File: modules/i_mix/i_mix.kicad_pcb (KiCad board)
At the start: 2 copper layers, 30.5 x 68.6 mm, 4 parts

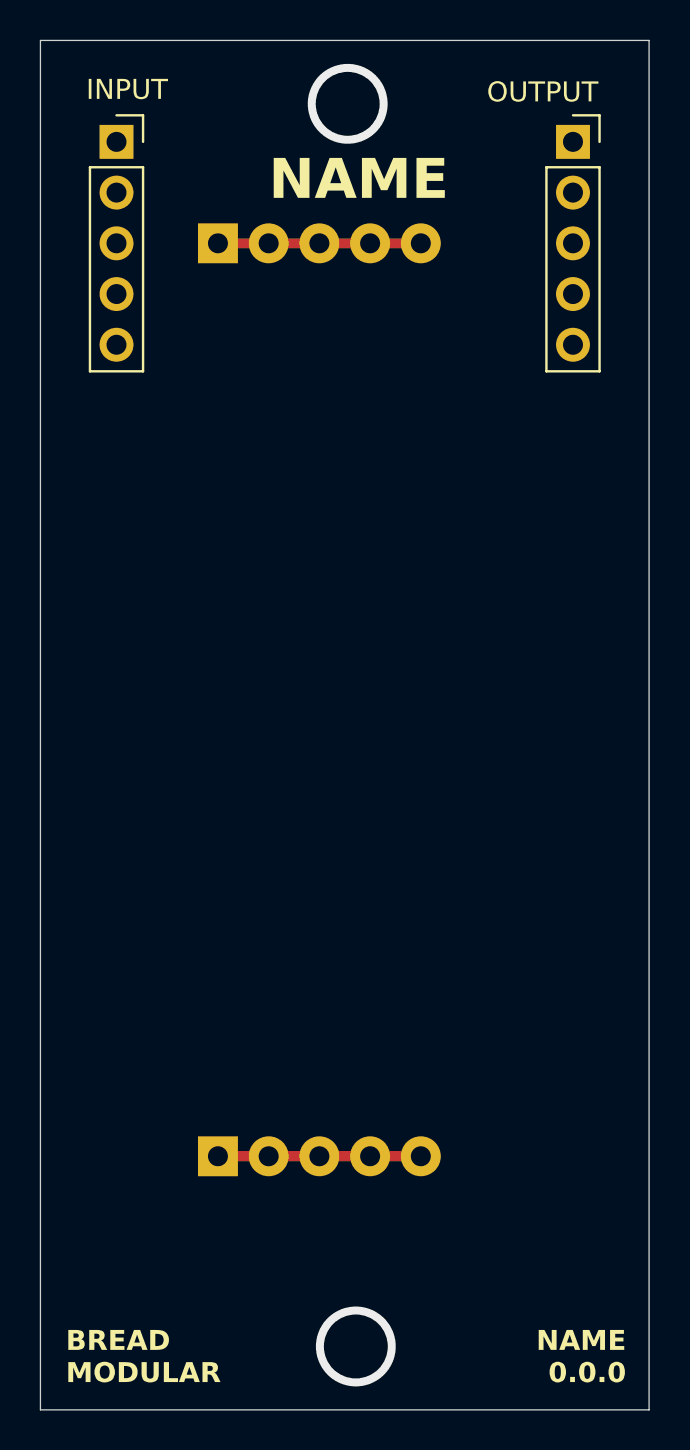
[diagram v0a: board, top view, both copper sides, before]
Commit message: Add production files
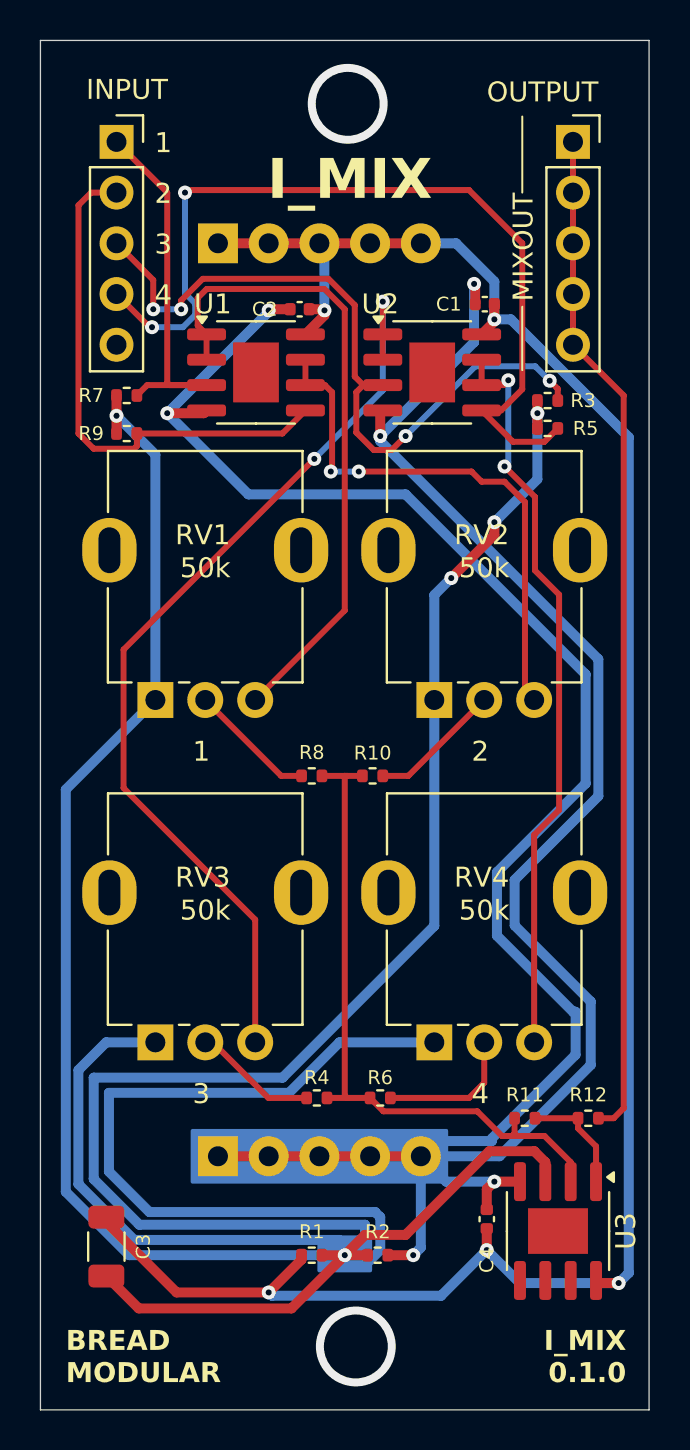
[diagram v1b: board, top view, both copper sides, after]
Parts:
- added C1: 0.1uf, Capacitor_SMD:C_0402_1005Metric, F.Cu at (69.2, 53.8)
- added C2: 0.1uf, Capacitor_SMD:C_0402_1005Metric, F.Cu at (60.0, 54.1)
- added C3: 100uf, Capacitor_SMD:C_1206_3216Metric, F.Cu at (50.3, 101.0)
- added C4: 0.1uf, Capacitor_SMD:C_0402_1005Metric, F.Cu at (69.3, 99.7)
- added R1: 1k, Resistor_SMD:R_0402_1005Metric, F.Cu at (60.6, 101.5)
- added R10: 200k, Resistor_SMD:R_0402_1005Metric, F.Cu at (63.6, 77.5)
- added R11: 200k, Resistor_SMD:R_0402_1005Metric, F.Cu at (71.2, 94.6)
- added R12: 1k, Resistor_SMD:R_0402_1005Metric, F.Cu at (74.4, 94.6)
- added R2: 1k, Resistor_SMD:R_0402_1005Metric, F.Cu at (63.9, 101.5)
- added R3: 1M, Resistor_SMD:R_0402_1005Metric, F.Cu at (72.4, 58.7)
- added R4: 200k, Resistor_SMD:R_0402_1005Metric, F.Cu at (60.8, 93.6)
- added R5: 1M, Resistor_SMD:R_0402_1005Metric, F.Cu at (72.4, 60.1)
- added R6: 200k, Resistor_SMD:R_0402_1005Metric, F.Cu at (64.0, 93.6)
- added R7: 1M, Resistor_SMD:R_0402_1005Metric, F.Cu at (51.3, 58.4)
- added R8: 200k, Resistor_SMD:R_0402_1005Metric, F.Cu at (60.6, 77.5)
- added R9: 1M, Resistor_SMD:R_0402_1005Metric, F.Cu at (51.3, 60.3)
- added RV1: 50k, BreadModular_Pots:Potentiometer_RV09, F.Cu at (55.4, 66.7)
- added RV2: 50k, BreadModular_Pots:Potentiometer_RV09, F.Cu at (69.3, 66.7)
- added RV3: 50k, BreadModular_Pots:Potentiometer_RV09, F.Cu at (55.4, 83.8)
- added RV4: 50k, BreadModular_Pots:Potentiometer_RV09, F.Cu at (69.3, 83.8)
- added U1: MCP6002-xSN, Package_SO:SOIC-8-1EP_3.9x4.9mm_P1.27mm_EP2.29x3mm, F.Cu at (57.8, 57.3)
- added U2: MCP6002-xSN, Package_SO:SOIC-8-1EP_3.9x4.9mm_P1.27mm_EP2.29x3mm, F.Cu at (66.6, 57.3)
- added U3: MCP6002-xSN, Package_SO:SOIC-8-1EP_3.9x4.9mm_P1.27mm_EP2.29x3mm, F.Cu at (72.9, 100.3)
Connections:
- INPUT1 pad 1: unconnected-(INPUT1-Pin_1-Pad1) -> IN_1
- INPUT1 pad 2: unconnected-(INPUT1-Pin_2-Pad2) -> IN_2
- INPUT1 pad 3: unconnected-(INPUT1-Pin_3-Pad3) -> IN_3
- INPUT1 pad 4: unconnected-(INPUT1-Pin_4-Pad4) -> IN_4
- OUTPUT1 pad 1: unconnected-(OUTPUT1-Pin_1-Pad1) -> MIXOUT
- OUTPUT1 pad 2: unconnected-(OUTPUT1-Pin_2-Pad2) -> MIXOUT
- OUTPUT1 pad 3: unconnected-(OUTPUT1-Pin_3-Pad3) -> MIXOUT
- OUTPUT1 pad 4: unconnected-(OUTPUT1-Pin_4-Pad4) -> MIXOUT
- OUTPUT1 pad 5: unconnected-(OUTPUT1-Pin_5-Pad5) -> MIXOUT
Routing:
- net V_MID: track 0.00 -> 224.3 mm, vias 0 -> 5
- net GND: track 10.2 -> 160.5 mm, vias 0 -> 6
- net V_SUPPLY: track 10.2 -> 109.8 mm, vias 0 -> 5
- net MIXOUT: track 0.00 -> 50.9 mm
- net Net-(U2A--): track 0.00 -> 48.1 mm, vias 0 -> 2
- net IN_4: track 0.00 -> 43.8 mm, vias 0 -> 2
- net Net-(U2B--): track 0.00 -> 37.6 mm, vias 0 -> 2
- net IN_3: track 0.00 -> 36.5 mm, vias 0 -> 4
- net Net-(U3A--): track 0.00 -> 33.7 mm
- net Net-(U1A--): track 0.00 -> 32.7 mm
- net Net-(U1B--): track 0.00 -> 27.2 mm, vias 0 -> 2
- net IN_2: track 0.00 -> 26.4 mm
- net IN_1: track 0.00 -> 18.8 mm
- net Net-(R6-Pad1): track 0.00 -> 7.04 mm
- net Net-(R10-Pad1): track 0.00 -> 6.65 mm
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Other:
- board text added: "1"
- board text added: "2"
- board text added: "3"
- board text added: "4"
- board text added: "I_MIX"
- board text added: "I_MIX 0.1.0"
- board text added: "MIXOUT"
- board text removed: "NAME"
- board text removed: "NAME 0.0.0"
